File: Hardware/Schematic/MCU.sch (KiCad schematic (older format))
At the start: 14 parts

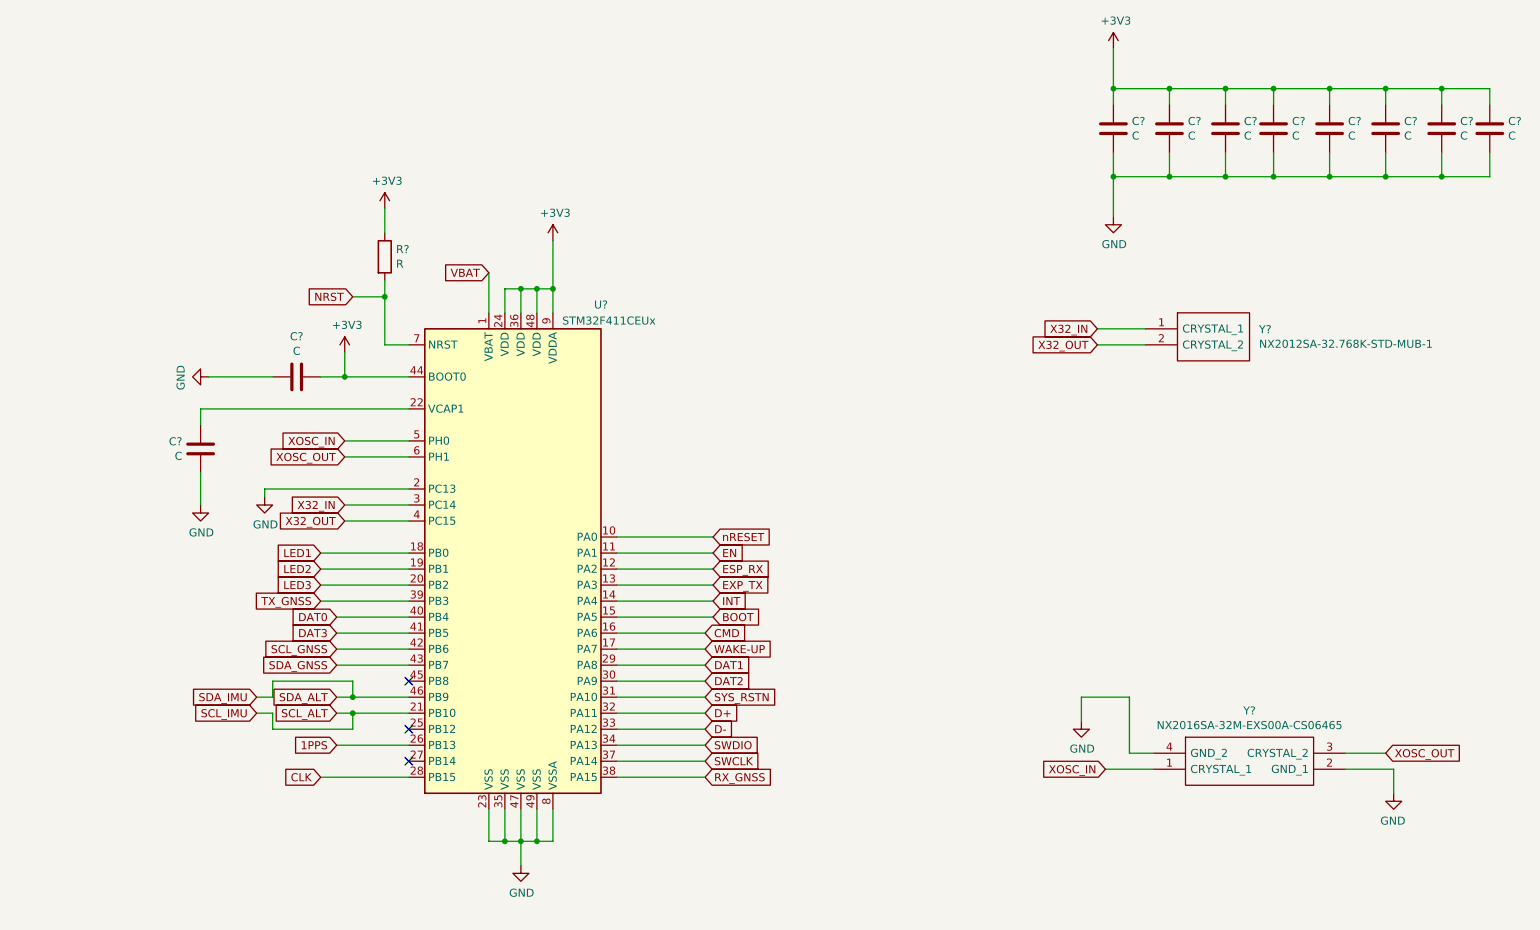
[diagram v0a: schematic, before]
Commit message: Add files via upload
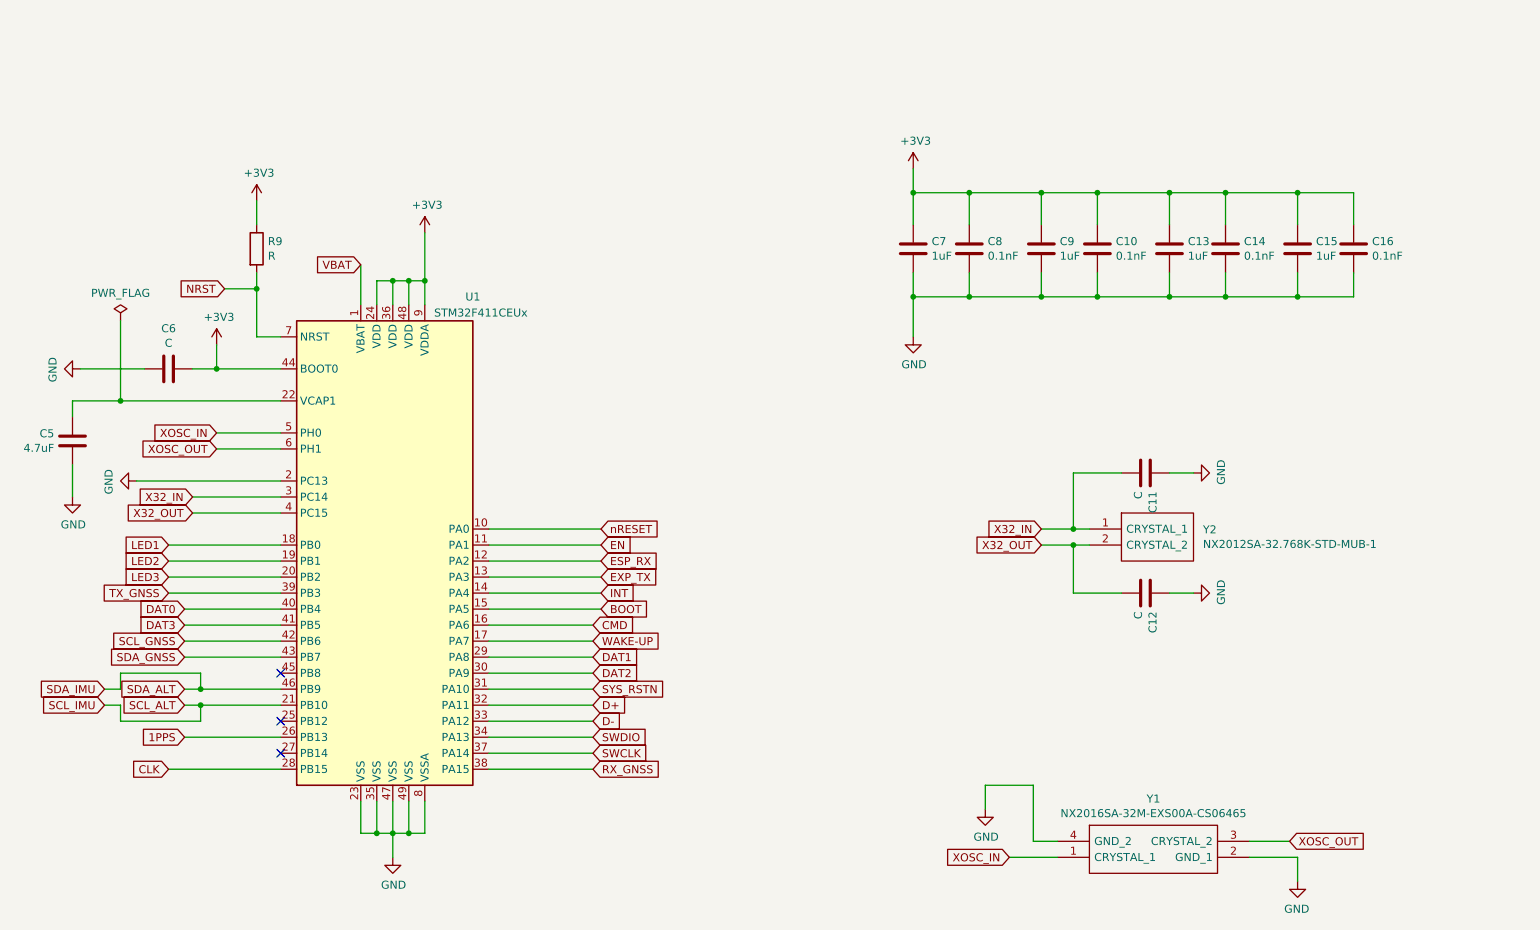
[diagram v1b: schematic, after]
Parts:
- removed C? (x6): C, symbol Device:C
- added C10, C14, C16: 0.1nF, Capacitor_SMD:C_0402_1005Metric, symbol Device:C
- added C11, C12: C, Capacitor_SMD:C_0402_1005Metric, symbol Device:C
- added C13, C15, C9: 1uF, Capacitor_SMD:C_0402_1005Metric, symbol Device:C
- C5: renamed from C?; value C -> 4.7uF; footprint (none) -> Capacitor_SMD:C_0402_1005Metric
- C6: renamed from C?; footprint (none) -> Capacitor_SMD:C_0402_1005Metric
- C7: renamed from C?; value C -> 1uF; footprint (none) -> Capacitor_SMD:C_0402_1005Metric
- C8: renamed from C?; value C -> 0.1nF; footprint (none) -> Capacitor_SMD:C_0402_1005Metric
- R9: renamed from R?; footprint (none) -> Resistor_SMD:R_0402_1005Metric
- gave numbers to parts that had none: 3
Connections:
- net +3V3: now also C10.1, C13.1, C14.1, C15.1, C16.1, C9.1
- net GND: now also C10.2, C11.1, C12.1, C13.2, C14.2, C15.2, C16.2, C9.2
- net X32_IN: now also C11.2
- net X32_OUT: now also C12.2
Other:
- moved on the sheet: C5, C6, C7, C8, R9, U1, Y1, Y2
